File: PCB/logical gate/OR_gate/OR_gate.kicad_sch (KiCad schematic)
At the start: 38 parts, among them J1 Conn_01x07, J2 Conn_01x07, Q1 P-MOS, Q10 N-MOS, Q11 P-MOS, Q12 N-MOS, Q2 N-MOS, Q3 P-MOS, Q4 N-MOS, Q5 P-MOS, Q6 N-MOS, Q7 P-MOS, Q8 N-MOS, Q9 P-MOS

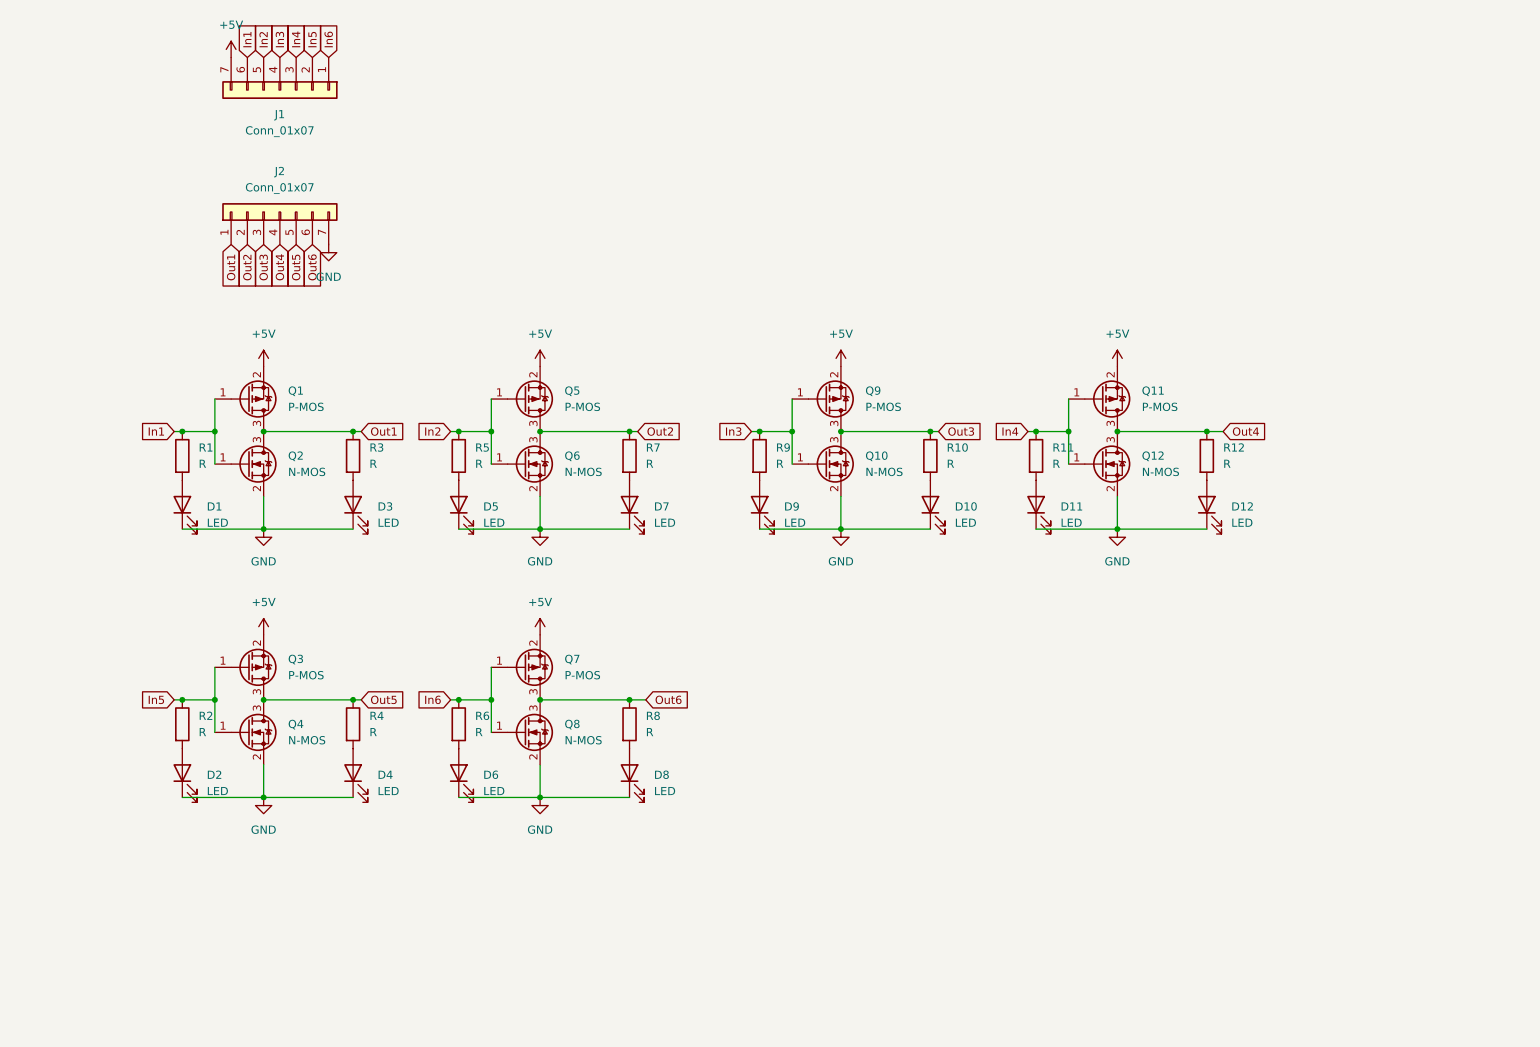
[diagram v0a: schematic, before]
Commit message: 20230309 1854
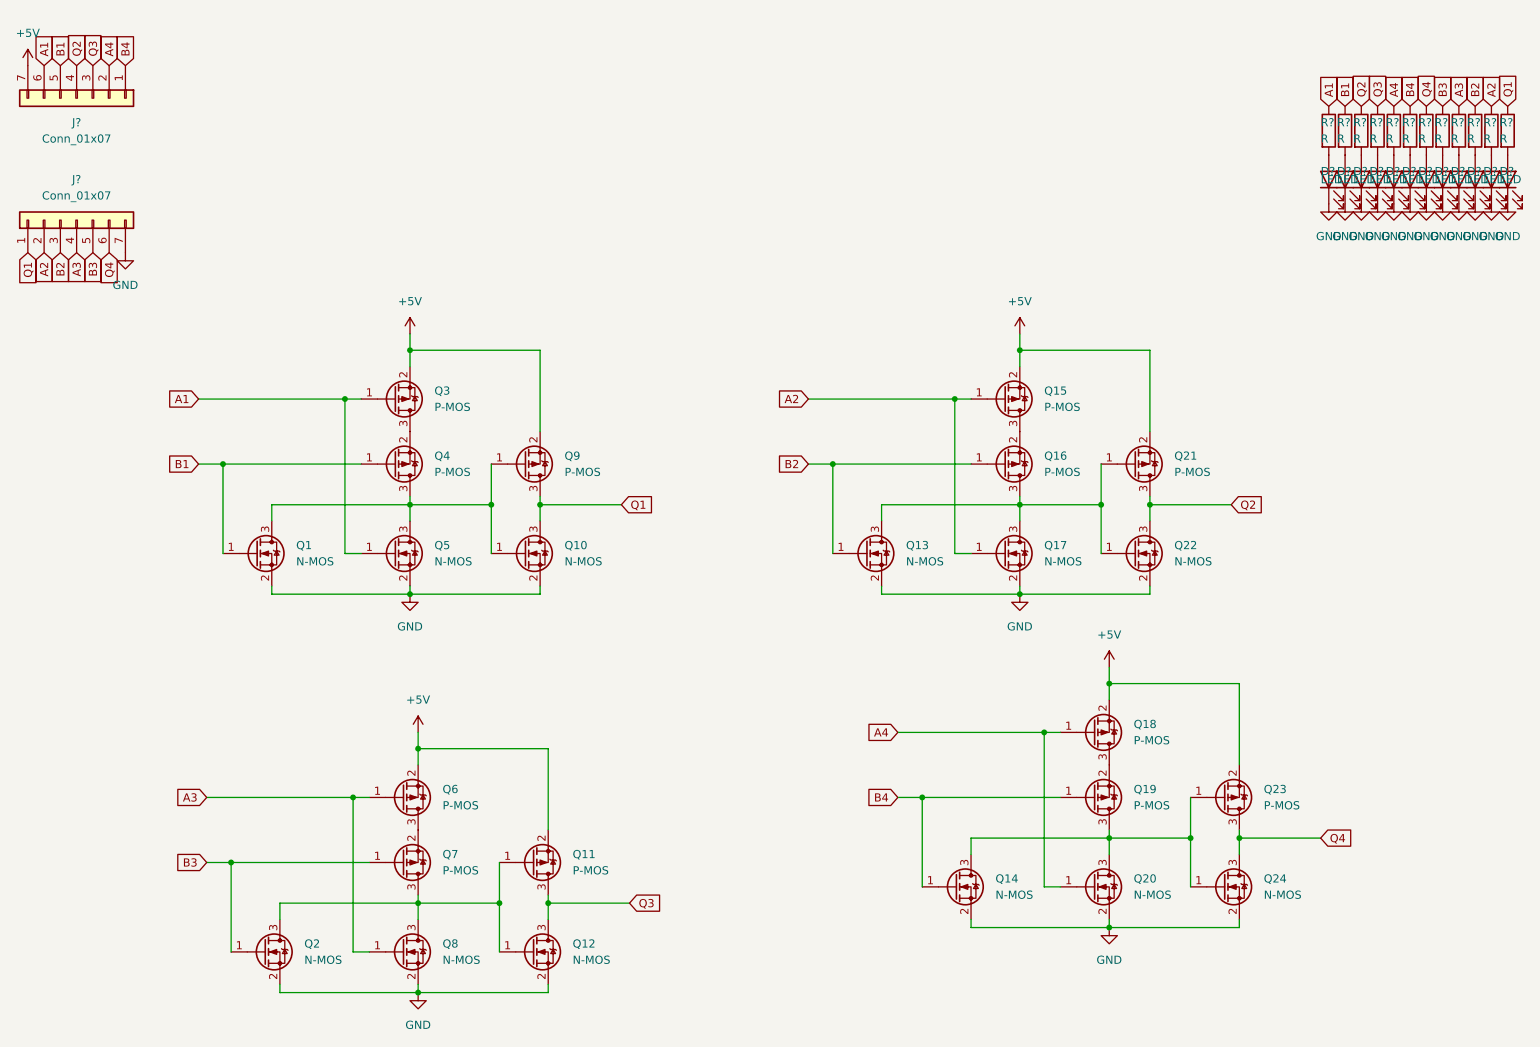
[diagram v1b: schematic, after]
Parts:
- removed D1, D10, D11, D12, D2, D3, D4, D5, D6, D7, D8, D9: LED, LED_SMD:LED_0805_2012Metric, symbol Device:LED
- removed J1, J2: Conn_01x07, Connector_PinHeader_2.54mm:PinHeader_1x07_P2.54mm_Vertical, symbol Connector_Generic:Conn_01x07
- removed Q1, Q5: P-MOS, Package_TO_SOT_SMD:SOT-23, symbol mos_sym:P-MOS
- removed Q4, Q6: N-MOS, Package_TO_SOT_SMD:SOT-23, symbol mos_sym:N-MOS
- removed R1, R10, R11, R12, R2, R3, R4, R5, R6, R7, R8, R9: R, Resistor_SMD:R_0805_2012Metric, symbol Device:R
- added D? (x12): LED, LED_SMD:LED_0805_2012Metric, symbol Device:LED
- added J? (x2): Conn_01x07, Connector_PinHeader_2.54mm:PinHeader_1x07_P2.54mm_Vertical, symbol Connector_Generic:Conn_01x07
- added Q1, Q13, Q14, Q17, Q20, Q22, Q24, Q5: N-MOS, Package_TO_SOT_SMD:SOT-23, symbol mos_sym:N-MOS
- added Q15, Q16, Q18, Q19, Q21, Q23, Q4, Q6: P-MOS, Package_TO_SOT_SMD:SOT-23, symbol mos_sym:P-MOS
- added R? (x12): R, Resistor_SMD:R_0805_2012Metric, symbol Device:R
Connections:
- net Out1 is gone; now on an unnamed net: Q2.3 (D)
- net Out6 is gone; now on an unnamed net: Q7.3 (D), Q8.3 (D)
- net +5V: now also J?.7 (Pin_7), Q15.2 (S), Q18.2 (S), Q21.2 (S), Q23.2 (S), Q6.2 (S); no longer Q7.2 (S)
- net GND: now also D?.1 (K), D?.1 (K), D?.1 (K), D?.1 (K), D?.1 (K), D?.1 (K), D?.1 (K), D?.1 (K), D?.1 (K), D?.1 (K), D?.1 (K), D?.1 (K), J?.7 (Pin_7), Q1.2 (S), Q13.2 (S), Q14.2 (S), Q17.2 (S), Q20.2 (S), Q22.2 (S), Q24.2 (S), Q5.2 (S)
- net In1 renamed B3
- net B3: now also Q7.1 (G), J?.5 (Pin_5), R?.1
- net In3: no longer names the net of Q10.1 (G), Q9.1 (G)
- net In3: now also Q1.3 (D), Q4.3 (D), Q5.3 (D)
- net In4: no longer names the net of Q11.1 (G), Q12.1 (G)
- net In5 renamed A1
- net A1: now also J?.6 (Pin_6), Q5.1 (G), R?.1
- net In6 renamed A3
- net A3: now also J?.4 (Pin_4), Q6.1 (G), R?.1; no longer Q7.1 (G)
- net Out3 renamed Q1
- net Q1: now also J?.1 (Pin_1), R?.1
- net Out4 renamed Q3
- net Q3: now also J?.3 (Pin_3), R?.1
- net Out5: no longer names the net of Q3.3 (D)
- net Out5: now also Q4.2 (S)
- new net: Q15.3 (D), Q16.2 (S)
- new net: D?.2 (A), R?.2 (x12)
- new net: Q13.3 (D), Q16.3 (D), Q17.3 (D), Q21.1 (G), Q22.1 (G)
- new net: Q6.3 (D), Q7.2 (S)
- new net: Q18.3 (D), Q19.2 (S)
- new net: Q14.3 (D), Q19.3 (D), Q20.3 (D), Q23.1 (G), Q24.1 (G)
- new net A2: J?.2 (Pin_2), Q15.1 (G), Q17.1 (G), R?.1
- new net A4: J?.2 (Pin_2), Q18.1 (G), Q20.1 (G), R?.1
- new net B1: J?.5 (Pin_5), Q1.1 (G), Q4.1 (G), R?.1
- new net B2: J?.3 (Pin_3), Q13.1 (G), Q16.1 (G), R?.1
- new net B4: J?.1 (Pin_1), Q14.1 (G), Q19.1 (G), R?.1
- new net Q2: J?.4 (Pin_4), Q21.3 (D), Q22.3 (D), R?.1
- new net Q4: J?.6 (Pin_6), Q23.3 (D), Q24.3 (D), R?.1
